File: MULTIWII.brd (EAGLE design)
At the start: 65.6 x 59.8 mm, 36 parts, among them IC1 MEGA8-PU, Q1 16MHz, Q2 BSS138, Q3 BSS138, U1 BMP180

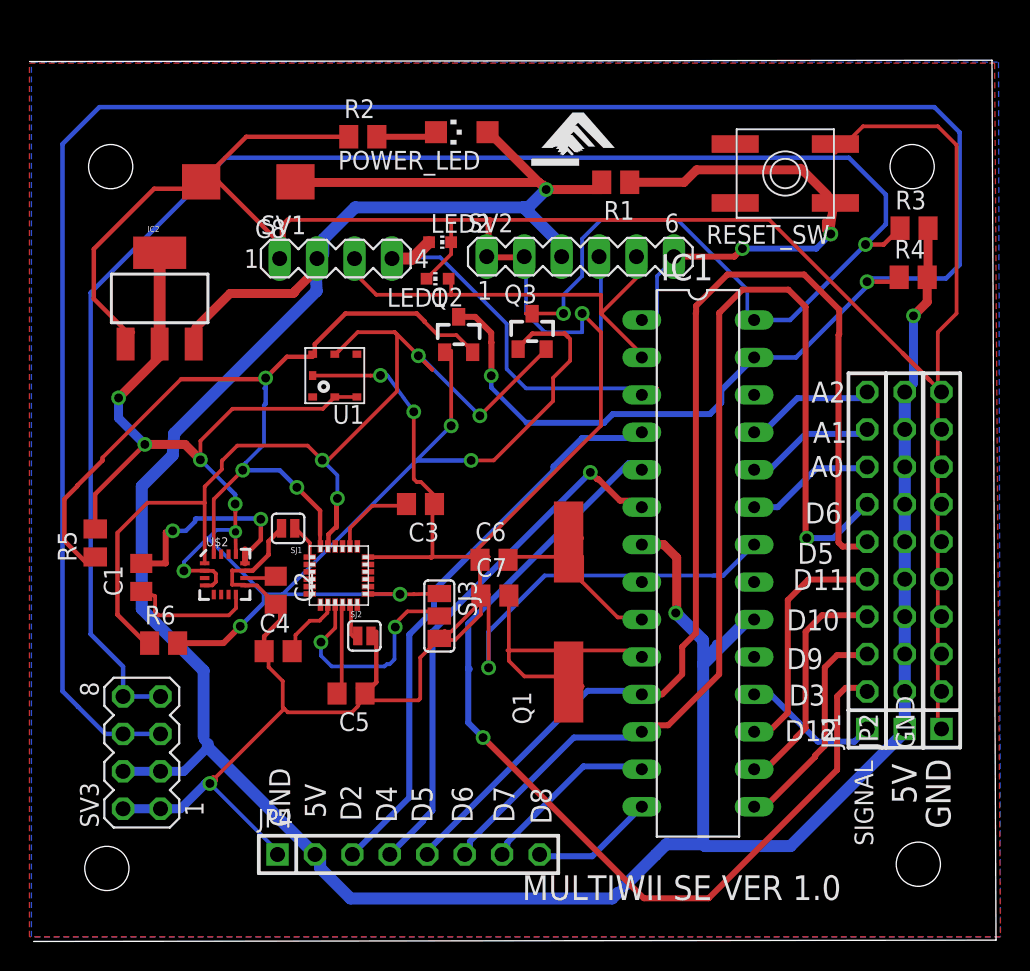
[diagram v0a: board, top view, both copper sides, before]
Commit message: modified:   MULTIWII.brd 	modified:   MULTIWII.sch
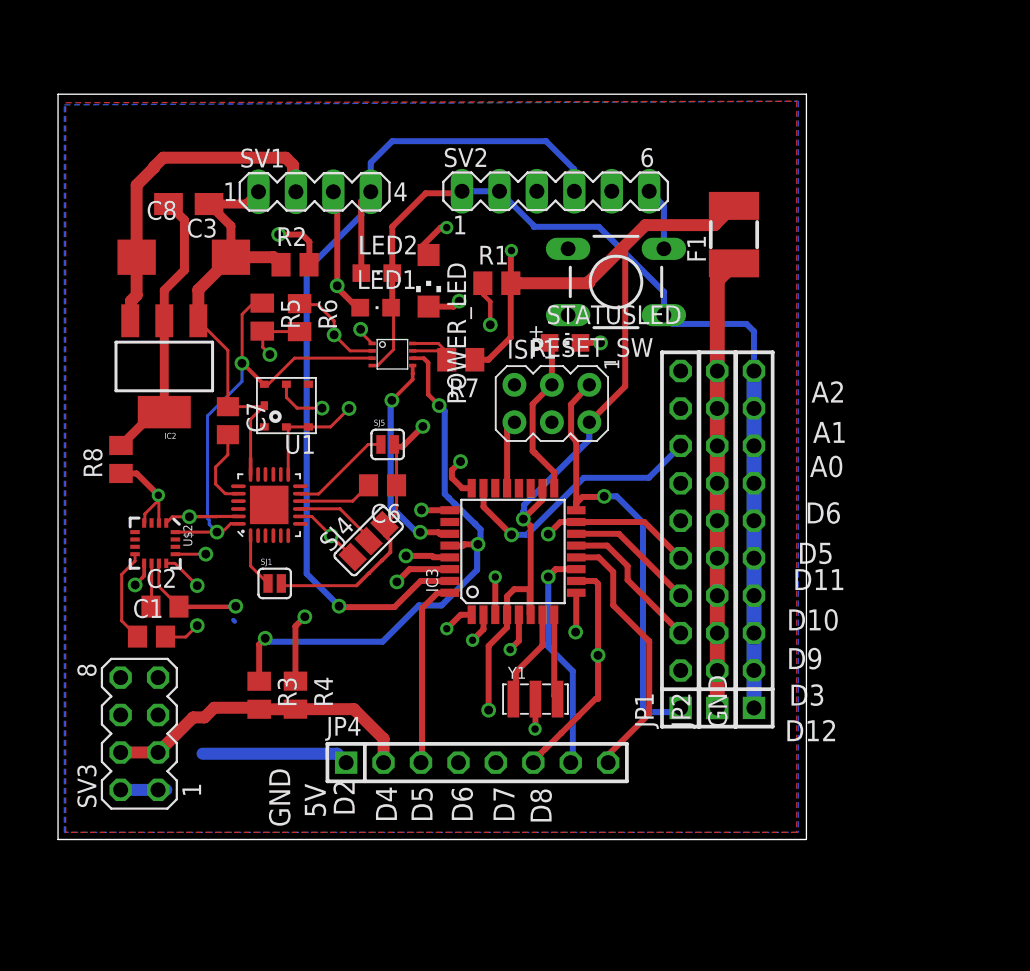
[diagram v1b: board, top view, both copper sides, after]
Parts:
- removed C4: 10nF, rcl:C0805
- removed C5: 0.1uF, rcl:C0805
- removed IC1: MEGA8-PU, avr-7:DIL28-3
- removed Q1: 16MHz, crystal:CSM-7X-DU
- removed Q2, Q3: BSS138, m-pad-2.1:SOT23
- removed SJ2: SOLDERJUMPERNC, Eagle-JeeLabs:SJ_2S
- removed SJ3: JUMPER, jumper:SJ_2
- removed U$1: MPU-6050, invensense:QFN.24.4X4
- added F1: (no value), m-pad-2.1:1812
- added IC3: MEGA8-AI, avr-7:TQFP32-08
- added ISP1: AVRISP-6, adafruit:AVRISP
- added PCA9306: (no value), SparkFun-DigitalIC:PSOP-8
- added R7, R8: 1K, rcl:M0805
- added SJ4: JUMPER, jumper:SJ_2
- added SJ5: SOLDERJUMPERNC, Eagle-JeeLabs:SJ_2S
- added STATUSLED: (no value), adafruit:CHIP-LED0805
- added U2: MPU-6000QFN-24, SparkFun-Sensors:QFN-24-TESTING
- added Y1: 16MHz, m-pad-2.1:RESONATOR_MURATA3
- C3: value 2.2nF -> (none); device rcl:C0805 -> rcl:A/3216-18R
- C6: value 22PF -> 0.1uF
- C7: value 22PF -> 2.2nF
- LED1, LED2: device led:CHIP-LED0603 -> adafruit:CHIPLED_0805
- RESET_SW: value SPST_TACT-EVQQ2 -> DTS-6; device adafruit:EVQ-Q2 -> switch-tact:DTS-6
- moved R3 54.6 mm to (25.1, 63.0), turned to 270 degrees
- moved R4 50.6 mm to (27.5, 63.0), turned to 270 degrees
- moved C3 25.7 mm to (20.3, 96.3)
- moved R6 23.9 mm to (27.8, 88.6), turned to 270 degrees
- moved C7 21.7 mm to (23.0, 81.6), turned to 270 degrees
- moved R5 19.1 mm to (25.3, 88.7), turned to 270 degrees
- moved RESET_SW 13.6 mm to (49.3, 91.0)
- moved GND 12.8 mm to (58.6, 73.6)
- moved JP2 12.8 mm to (56.2, 73.6)
- moved JP1 12.7 mm to (53.7, 73.6)
- moved R1 10.6 mm to (41.2, 91.0), turned to 0 degrees
- moved POWER_LED 10.3 mm to (36.6, 91.1), turned to 180 degrees
- moved R2 9.82 mm to (27.5, 92.2)
- moved C6 9.10 mm to (33.4, 77.2), turned to 180 degrees
- moved JP4 7.78 mm to (39.9, 58.4)
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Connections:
- net N$5 renamed C1
- removed net N$10: C5.2, U$1.10
- removed net N$3: SJ3.2, U$1.9
- removed net N$4: C3.2, U$1.20
- new net AD0: SJ4.2, U2.9
- new net AUXCL: U2.7
- new net AUXDA: U2.6
- new net CLKOUT: U2.22
- new net INT: U2.12
- new net N$16: SJ5.1, U2.11
- new net N$17: SJ1.1, U2.1
- new net N$18: C6.2, U2.10
- new net RAW: F1.1, JP2.1, JP2.10, JP2.2, JP2.3, JP2.4, JP2.5, JP2.6, JP2.7, JP2.8, JP2.9, SV2.3
- new net SCK: IC3.17, ISP1.3, STATUSLED.A
- net 3.3V: now also PCA9306.1, R8.1, SJ4.1, U2.13, U2.8; no longer IC2.2, IC2.4, Q2.1, Q3.1, SJ3.1, U$1.13
- net 5V: now also F1.2, IC3.18, IC3.4, IC3.6, ISP1.2, R7.1; no longer IC1.20, IC1.7, JP2.1, JP2.10, JP2.2, JP2.3, JP2.4, JP2.5, JP2.6, JP2.7, JP2.8, JP2.9, SV2.3
- net A0: now also IC3.23; no longer IC1.23
- net A1: now also IC3.24; no longer IC1.24
- net A2: now also IC3.25; no longer IC1.25
- net D10: now also IC3.14; no longer IC1.16
- net D11: now also IC3.15, ISP1.4; no longer IC1.17
- net D12: now also IC3.16, ISP1.1; no longer IC1.18
- net D2: now also IC3.32; no longer IC1.4
- net D3: now also IC3.1; no longer IC1.5
- net D4: now also IC3.2; no longer IC1.6
- net D5: now also IC3.9; no longer IC1.11
- net D6: now also IC3.10; no longer IC1.12
- net D7: now also IC3.11; no longer IC1.13
- net D8: now also IC3.12; no longer IC1.14
- net D9: now also IC3.13; no longer IC1.15
- net GND: now also C3.-, IC3.21, IC3.3, IC3.5, ISP1.6, PCA9306.4, RESET_SW.1, SJ4.3, SJ5.2, STATUSLED.C, U2.18, Y1.2; no longer C3.1, C4.1, C5.1, IC1.22, IC1.8, RESET_SW.A, SJ2.2, SJ3.3, U$1.18
- net N$1: now also C7.2, U2.20; no longer SJ1.1, U$1.1
- net N$11: now also IC3.8, Y1.3; no longer C7.2, IC1.10, Q1.1
- net N$2: now also C3.+, IC2.2, IC2.4, R8.2; no longer SJ2.1, U$1.11
- net N$6: now also IC3.7, Y1.1; no longer C6.2, IC1.9, Q1.2
- net N$9: now also PCA9306.7, PCA9306.8, R7.2; no longer C4.2, U$1.8
- net RESET: now also IC3.29, ISP1.5, RESET_SW.3; no longer IC1.1, RESET_SW.B
- net RX: now also IC3.30; no longer IC1.2
- net SCL: now also PCA9306.2, U2.23; no longer Q3.2, U$1.23
- net SCL0: now also IC3.28, PCA9306.6; no longer IC1.28, Q3.3
- net SDA: now also PCA9306.3, U2.24; no longer Q2.2, U$1.24
- net SDA0: now also IC3.27, PCA9306.5; no longer IC1.27, Q2.3
- net TX: now also IC3.31; no longer IC1.3
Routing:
- net SDA0: track 163.2 -> 47.4 mm, vias 2 -> 3
- net GND: track 313.0 -> 200.1 mm, vias 5 -> 7
- net 5V: track 236.1 -> 144.1 mm, vias 3 -> 4
- net SCL0: track 130.6 -> 50.4 mm, vias 2 -> 3
- net 3.3V: track 125.7 -> 65.3 mm, vias 10 -> 6
- net RAW: track 0.00 -> 51.5 mm
- net D5: track 78.7 -> 30.5 mm, vias 0 -> 1
- net D6: track 75.8 -> 30.3 mm
- net D3: track 64.5 -> 20.8 mm
- net SCL: track 73.2 -> 38.9 mm, vias 4 -> 3
- net RX: track 30.2 -> 59.4 mm, vias 0 -> 2
- net SDA: track 62.6 -> 34.4 mm, vias 3 -> 2
- net TX: track 36.5 -> 63.5 mm, vias 0 -> 1
- net D2: track 39.3 -> 12.8 mm
- net D4: track 36.5 -> 10.8 mm
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- added copper zone on layer 1, net 5V
- removed copper zone on layer 1, net GND
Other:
- board size 65.6 x 59.8 mm -> 50.8 x 50.6 mm
- board text removed: "MULTIWII SE VER 1.0"
- board text removed: "SIGNAL"
- board text removed: "^"
- board text removed: "_"
